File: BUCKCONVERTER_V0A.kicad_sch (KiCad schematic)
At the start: 1 part

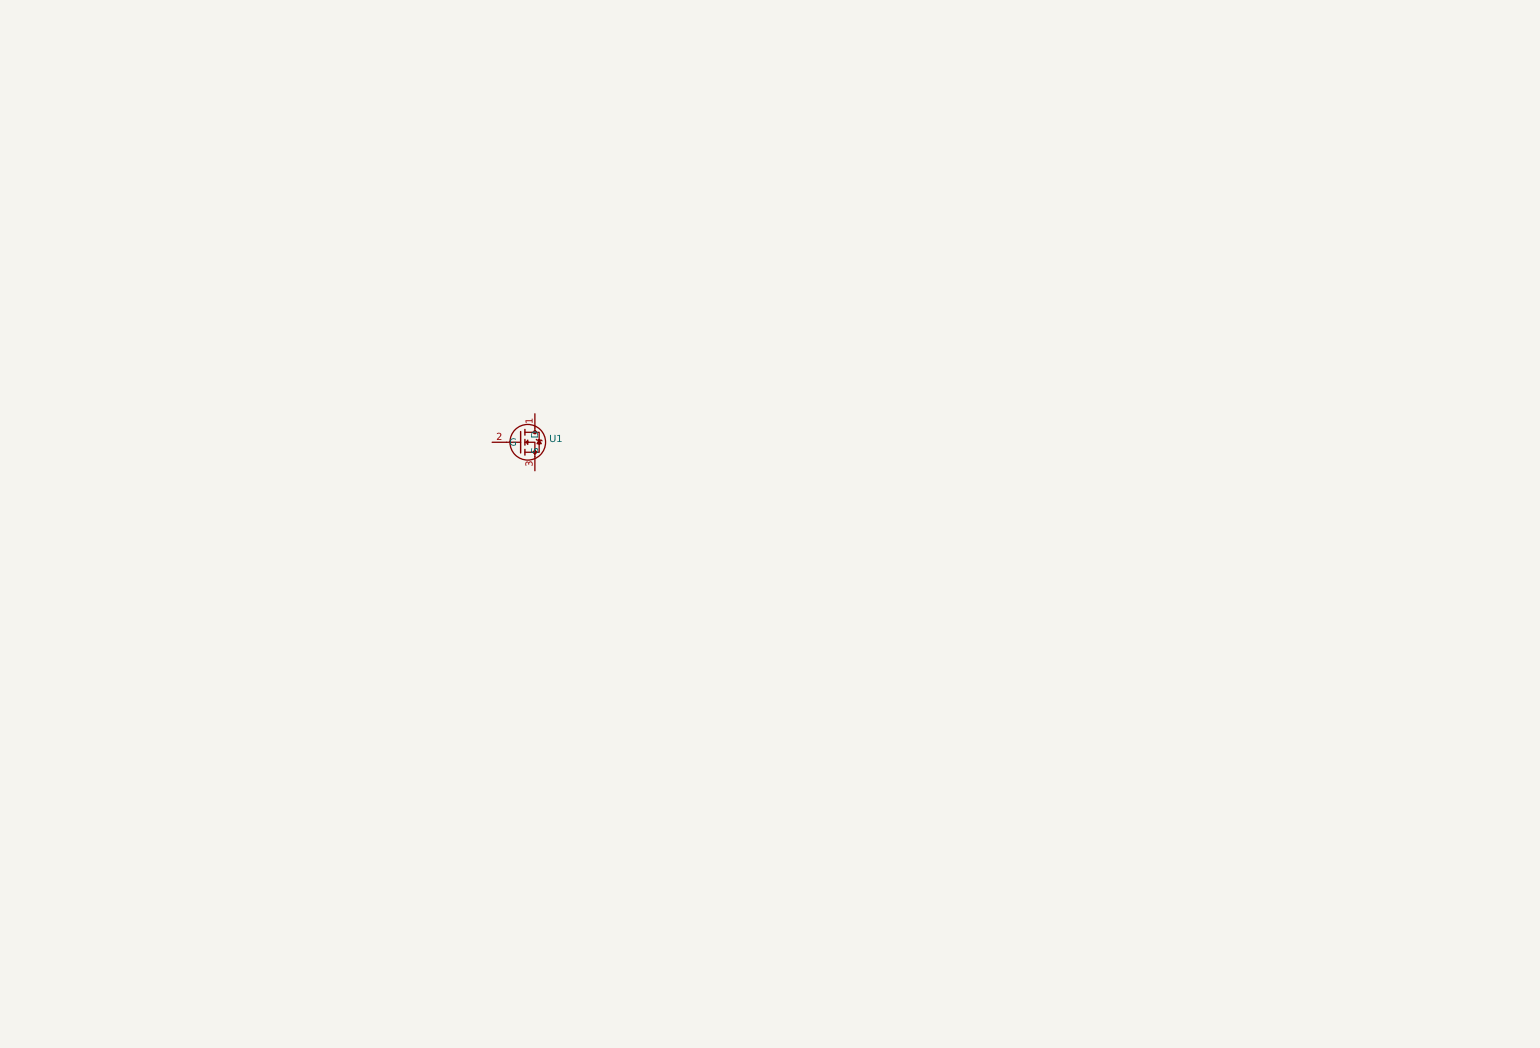
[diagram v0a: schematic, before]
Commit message: Add files via upload
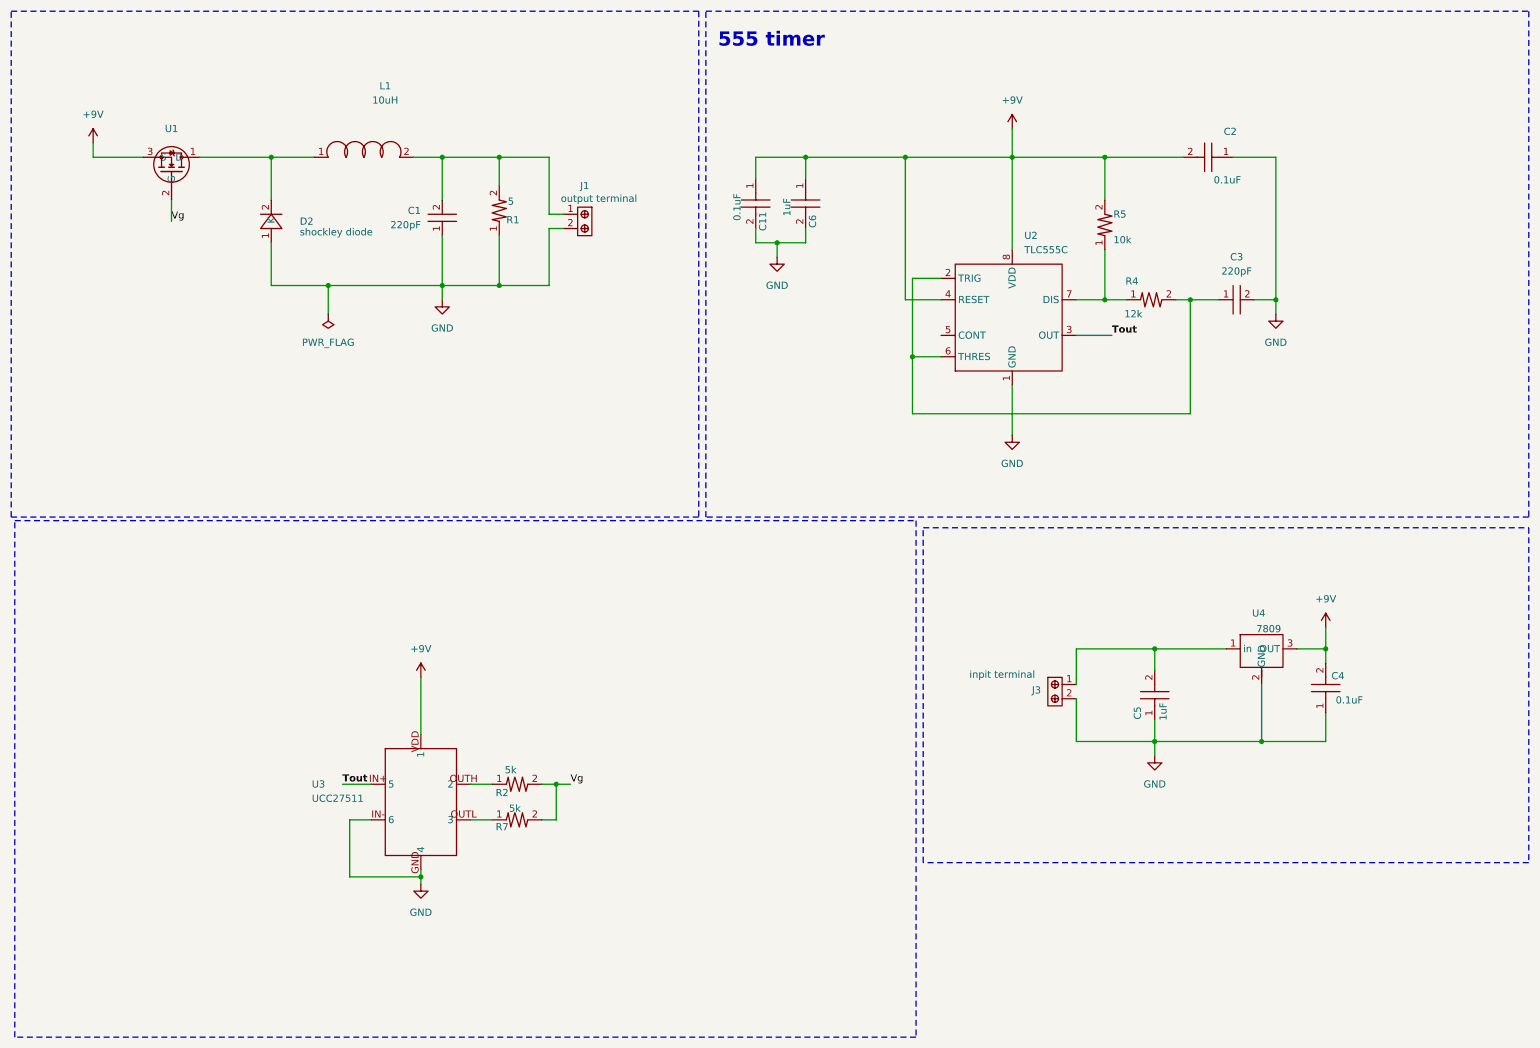
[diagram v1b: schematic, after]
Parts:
- added C1, C3: 220pF, BuckConverter_V0A:C0603, symbol buck_converter:C0603_220pF
- added C11: 0.1uF, BuckConverter_V0A:C0603, symbol buck_converter:CO6O3_1uF
- added C2, C4: 0.1uF, BuckConverter_V0A:C0603, symbol buck_converter:CO6O3_0.1uF
- added C5, C6: 1uF, BuckConverter_V0A:C0603, symbol buck_converter:CO6O3_1uF
- added D2: shockley diode, Diode_SMD:D_0201_0603Metric, symbol buck_converter:diode
- added J1: output terminal, BuckConverter_V0A:terminal_2x1, symbol buck_converter:terminal_2x1
- added J3: inpit terminal, BuckConverter_V0A:terminal_2x1, symbol buck_converter:terminal_2x1
- added L1: 10uH, BuckConverter_V0A:Inductor, symbol buck_converter:INDUCTOR
- added R1: 5, BuckConverter_V0A:R0603, symbol buck_converter:R0603_10K
- added R2, R7: 5k, BuckConverter_V0A:R0603, symbol buck_converter:R0603_10K
- added R4: 12k, BuckConverter_V0A:R0603, symbol buck_converter:R0603_10K
- added R5: 10k, BuckConverter_V0A:R0603, symbol buck_converter:R0603_10K
- added U2: TLC555C, BuckConverter_V0A:SOIC_8, symbol buck_converter:TLC555C
- added U3: UCC27511, BuckConverter_V0A:UCC, symbol buck_converter:UCC27511
- added U4: 7809, BuckConverter_V0A:7809, symbol buck_converter:7809
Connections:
- net at U1.1 (D): now also D2.2 (K), L1.1
- net Vg: now reaches U1.2 (G)
- net Vg: now also R2.2, R7.2
- net +9V: now reaches U1.3 (S)
- net +9V: now also C11.1, C2.2, C4.2, C6.1, R5.2, U2.4 (RESET), U2.8 (VDD), U3.VDD (1), U4.3 (OUT)
- new net: R4.1, R5.1, U2.7 (DIS)
- new net: C5.2, J3.1, U4.1 (in)
- new net: C1.2, J1.1, L1.2, R1.2
- new net: R7.1, U3.OUTL (3)
- new net: R2.1, U3.OUTH (2)
- new net: C3.1, R4.2, U2.2 (TRIG), U2.6 (THRES)
- new net GND: C1.1, C11.2, C2.1, C3.2, C4.1, C5.1, C6.2, D2.1, J1.2, J3.2, R1.1, U2.1 (GND), U3.GND (4), U3.IN- (6), U4.2 (GND)
- new net Tout: U2.3 (OUT), U3.IN+ (5)
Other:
- note added: "555 timer"
